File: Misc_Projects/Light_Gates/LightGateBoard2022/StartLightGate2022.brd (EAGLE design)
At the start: 38.1 x 47.9 mm, 6 parts

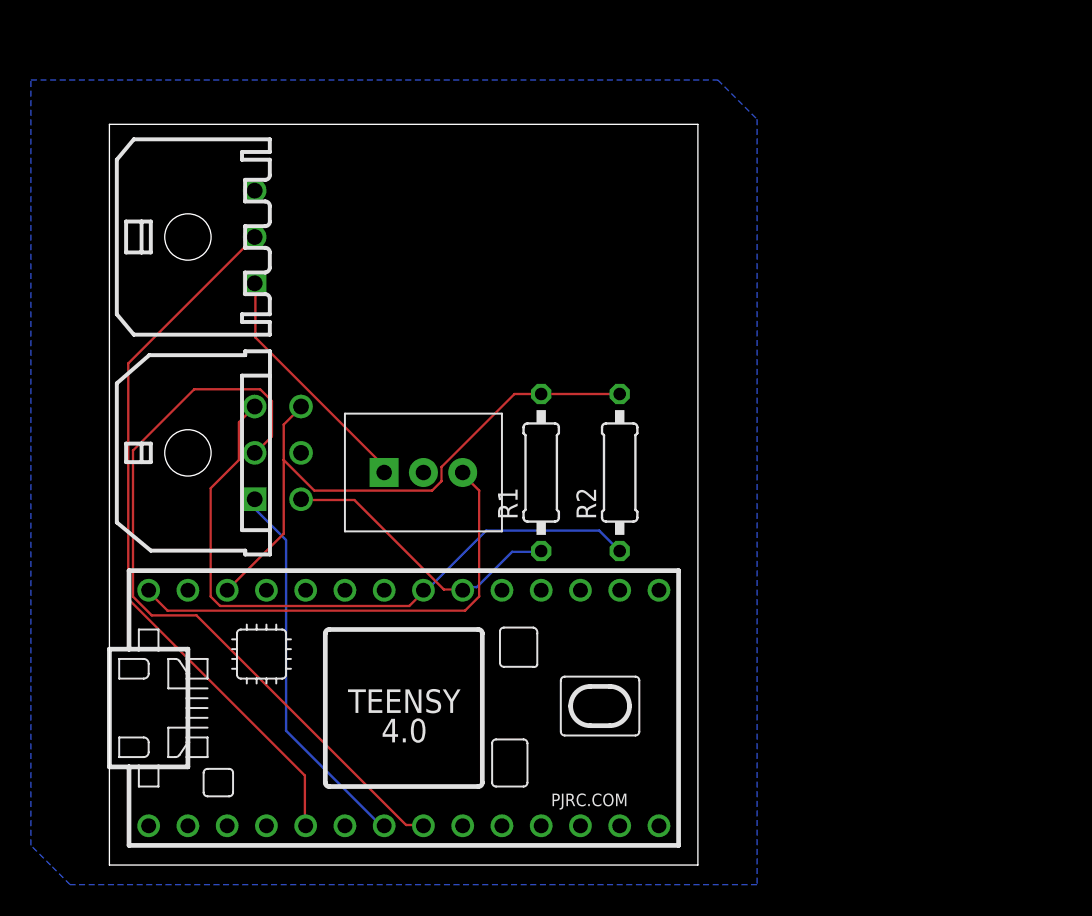
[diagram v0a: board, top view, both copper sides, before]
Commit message: Light Gate Updates
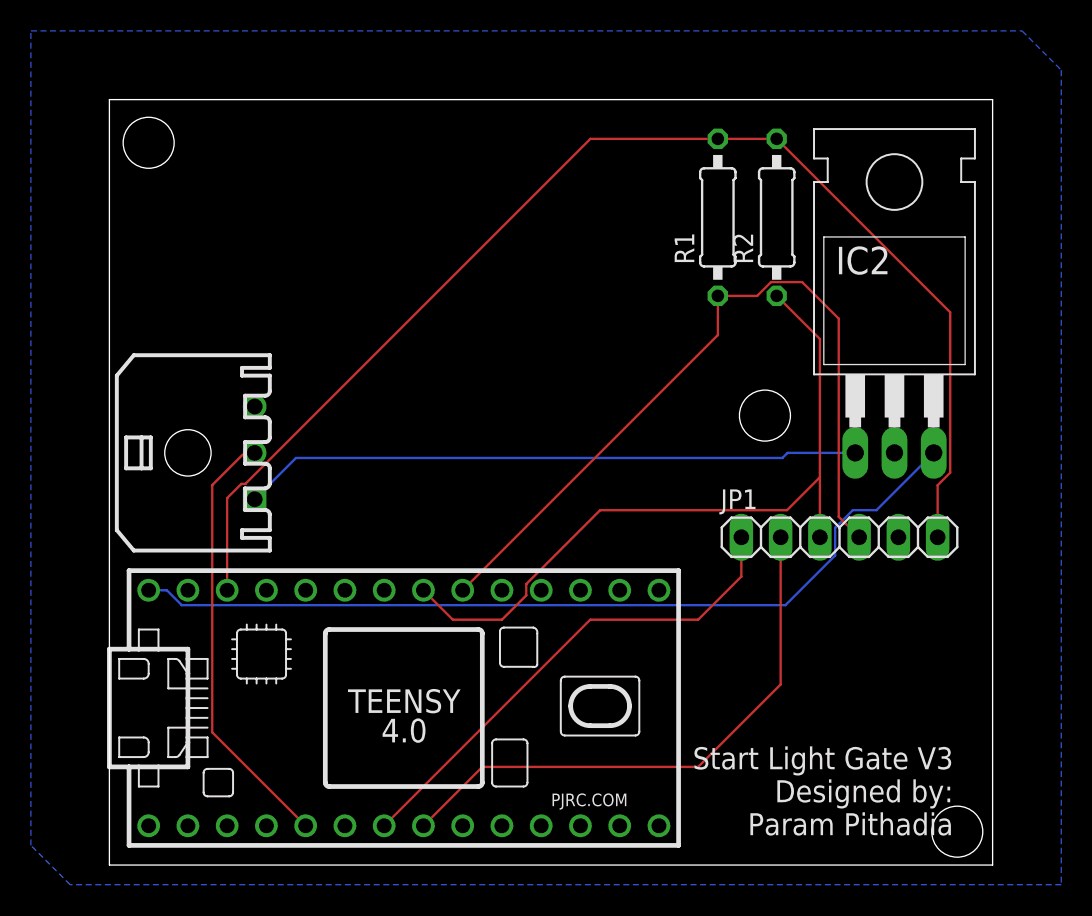
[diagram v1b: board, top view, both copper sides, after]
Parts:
- removed IC1: (no value), GTOR - Active Components:TO-220
- removed X1: (no value), GTOR - Microfit Connector:43045-0600
- added IC2: (no value), GTOR - Active Components:TO-220-H
- added JP1: (no value), GTOR - Connectors:1X06
- moved R1 20.1 mm to (39.4, 41.9)
- moved R2 19.4 mm to (43.2, 41.9)
- moved X2 14.0 mm to (5.08, 26.7)
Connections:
- net +3V3: now also JP1.6; no longer X1.P$6
- net +5V: now also IC2.3; no longer IC1.3
- net GND: now also IC2.2, JP1.5; no longer IC1.2, X1.P$5
- net INT: now also JP1.1; no longer X1.P$1
- net SCL: now also JP1.3; no longer X1.P$3
- net SDA: now also JP1.4; no longer X1.P$4
- net SHUT: now also JP1.2; no longer X1.P$2
- net VCC: now also IC2.1; no longer IC1.1
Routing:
- net +3V3: track 39.5 -> 81.9 mm
- net SDA: track 19.1 -> 49.8 mm
- net +5V: track 30.8 -> 56.3 mm
- net VCC: track 15.7 -> 40.1 mm
- net INPUT: track 46.2 -> 28.2 mm
- net SHUT: track 49.2 -> 36.4 mm
- net INT: track 24.7 -> 32.3 mm
- net SCL: track 42.9 -> 47.5 mm
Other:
- board size 38.1 x 47.9 mm -> 57.1 x 49.5 mm
